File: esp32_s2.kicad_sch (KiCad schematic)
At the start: 15 parts, among them U3 ESP32-S2-MINI-2U-N4

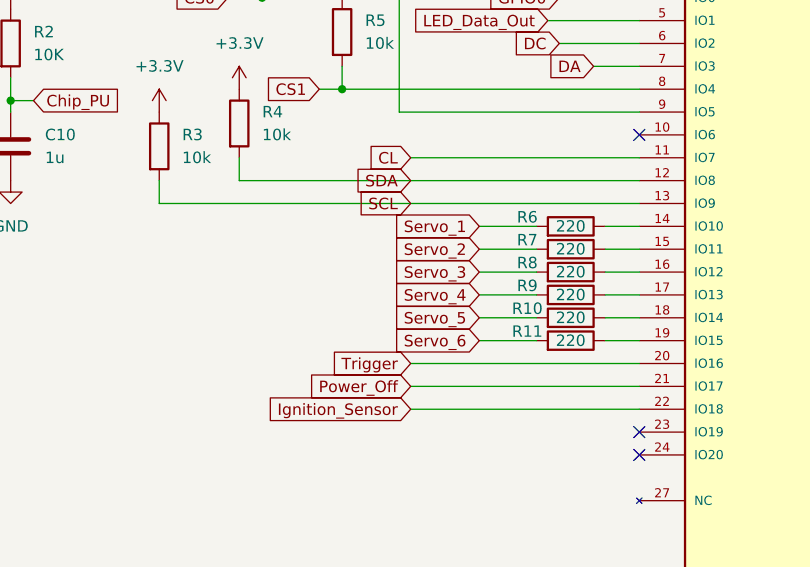
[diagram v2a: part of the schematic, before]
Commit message: update
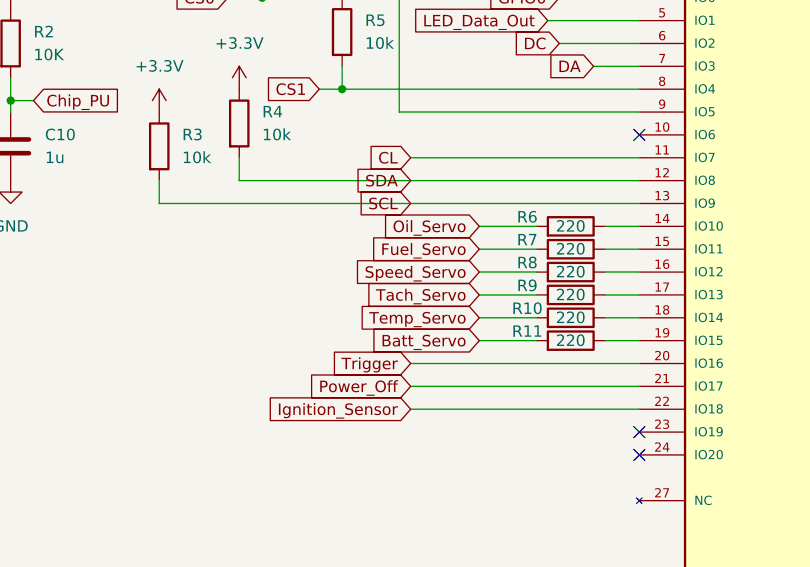
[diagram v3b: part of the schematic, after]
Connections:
- net Servo_1 renamed Oil_Servo
- net Servo_2 renamed Fuel_Servo
- net Servo_3 renamed Speed_Servo
- net Servo_4 renamed Tach_Servo
- net Servo_5 renamed Temp_Servo
- net Servo_6 renamed Batt_Servo
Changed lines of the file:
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@@
 		)
 	)
-	(global_label "Servo_4"
+	(global_label "Tach_Servo"
 		(shape input)
 		(at 69.85 76.2 180)
@@
 		)
 		(property "Intersheetrefs" "${INTERSHEET_REFS}"
-			(at 59.4868 76.2 0)
+			(at 56.3421 76.2 0)
 			(hide yes)
 			(show_name no)
@@
 		)
 	)
-	(global_label "Servo_5"
+	(global_label "Temp_Servo"
 		(shape input)
 		(at 69.85 78.74 180)
@@
 		)
 		(property "Intersheetrefs" "${INTERSHEET_REFS}"
-			(at 59.4868 78.74 0)
+			(at 55.7978 78.74 0)
 			(hide yes)
 			(show_name no)
@@
 		)
 	)
-	(global_label "Servo_2"
+	(global_label "Fuel_Servo"
 		(shape input)
 		(at 69.85 71.12 180)
@@
 		)
 		(property "Intersheetrefs" "${INTERSHEET_REFS}"
-			(at 59.4868 71.12 0)
+			(at 56.7049 71.12 0)
 			(hide yes)
 			(show_name no)
@@
 		)
 	)
-	(global_label "Servo_6"
+	(global_label "Batt_Servo"
 		(shape input)
 		(at 69.85 81.28 180)
@@
 		)
 		(property "Intersheetrefs" "${INTERSHEET_REFS}"
-			(at 59.4868 81.28 0)
+			(at 56.8259 81.28 0)
 			(hide yes)
 			(show_name no)
@@
 		)
 	)
-	(global_label "Servo_3"
+	(global_label "Speed_Servo"
 		(shape input)
 		(at 69.85 73.66 180)
@@
 		)
 		(property "Intersheetrefs" "${INTERSHEET_REFS}"
-			(at 59.4868 73.66 0)
+			(at 55.0116 73.66 0)
 			(hide yes)
 			(show_name no)
@@
 		)
 	)
-	(global_label "Servo_1"
+	(global_label "Oil_Servo"
 		(shape input)
 		(at 69.85 68.58 180)
@@
 		)
 		(property "Intersheetrefs" "${INTERSHEET_REFS}"
-			(at 59.4868 68.58 0)
-			(hide yes)
-			(show_name no)
+			(at 58.0958 68.58 0)
+			(hide yes)
+			(show_name no)
